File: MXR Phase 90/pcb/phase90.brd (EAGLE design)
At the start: 59 x 87.8 mm, 58 parts, among them IC1 TL072, IC2 TL074, J1 POWER_JACK, Q1 2N5457, Q2 2N5457, Q3 2N5457, Q4 2N5457, Q5 2N3906-, X1 2510-

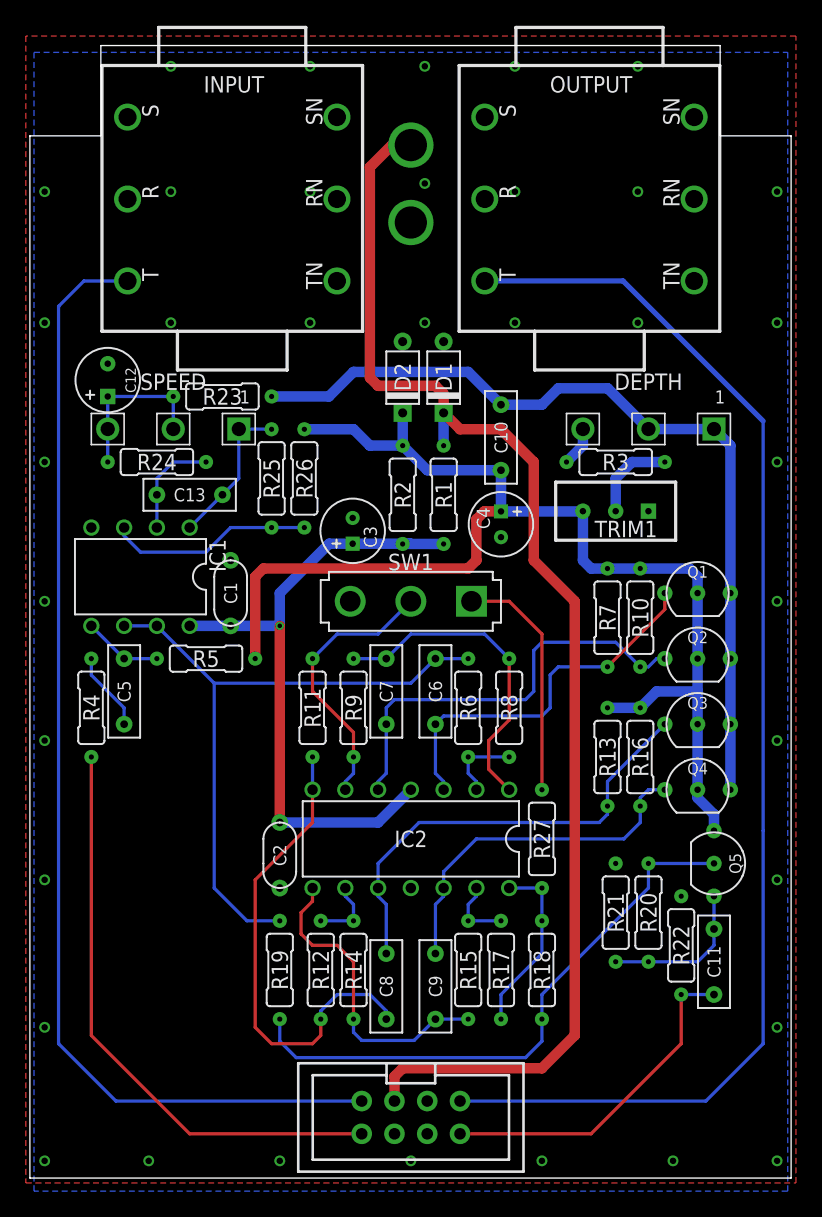
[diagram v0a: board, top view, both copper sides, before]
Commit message: 20171216
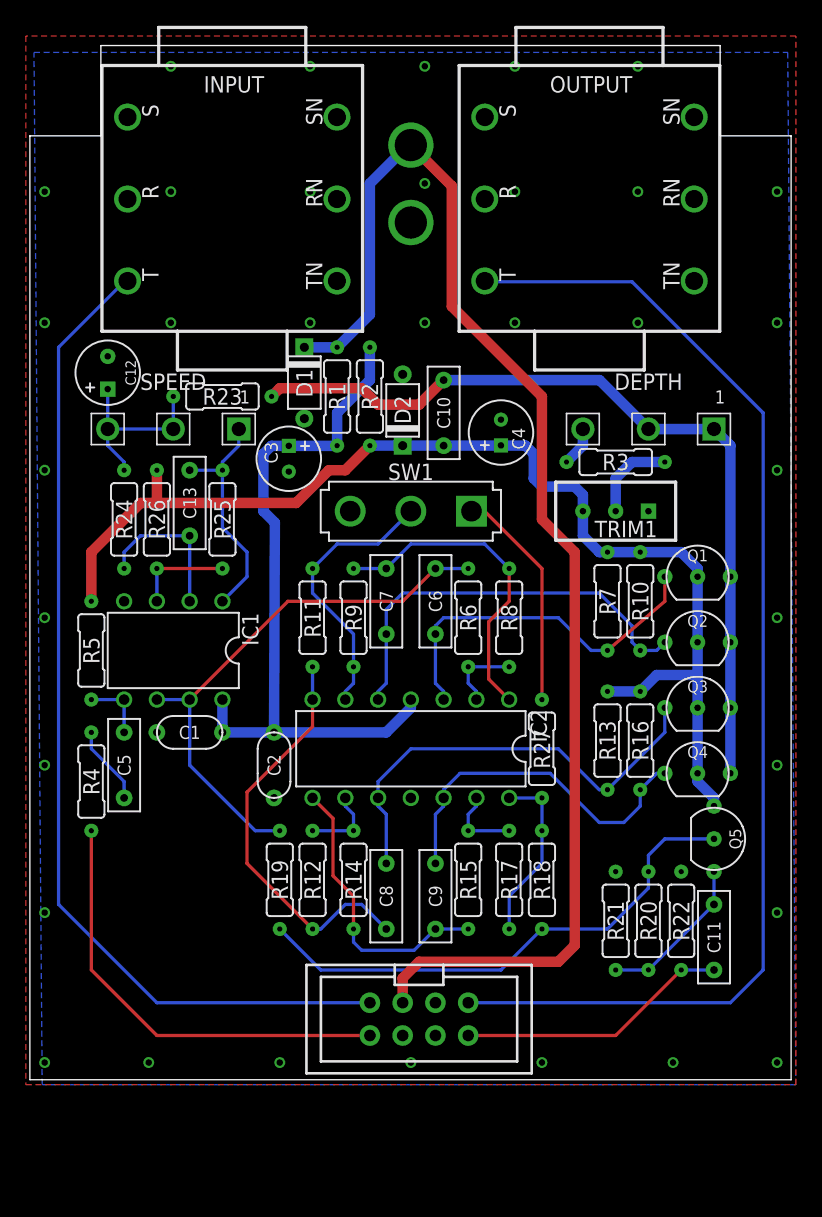
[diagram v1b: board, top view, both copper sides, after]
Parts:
- moved R26 11.9 mm to (9.53, 36.2)
- moved C1 11.3 mm to (12.1, 19.7), turned to 180 degrees
- moved R1 11.2 mm to (23.5, 45.7)
- moved D1 10.8 mm to (21.0, 46.8), turned to 270 degrees
- moved R5 8.91 mm to (4.45, 26.0), turned to 90 degrees
- moved R2 8.03 mm to (26.0, 45.7), turned to 270 degrees
- moved X1 7.65 mm to (29.8, -2.54)
- moved C3 7.47 mm to (19.7, 40.9), turned to 270 degrees
- moved C4 7.11 mm to (36.2, 42.9), turned to 90 degrees
- moved R12 7.01 mm to (21.6, 8.26)
- moved R17 7.01 mm to (36.8, 8.26)
- moved C2 7.00 mm to (18.6, 17.1)
- moved R14 6.99 mm to (24.8, 8.26)
- moved R15 6.99 mm to (33.7, 8.26)
- moved R18 6.99 mm to (39.4, 8.26)
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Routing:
- net IN: track 45.7 -> 34.5 mm
- net N$2: track 88.6 -> 77.9 mm
- net N$6: track 51.3 -> 42.5 mm
- net VB: track 99.0 -> 90.2 mm
- net N$15: track 15.9 -> 7.62 mm
- net N$4: track 99.7 -> 92.9 mm
- net N$19: track 11.8 -> 18.0 mm
- net N$14: track 37.3 -> 31.8 mm
- net OUT: track 26.4 -> 21.2 mm
- net N$24: track 45.4 -> 40.7 mm
- net N$26: track 8.15 -> 12.0 mm
- net VR: track 51.5 -> 55.2 mm, vias 1 -> 0
- net +9V: track 102.0 -> 104.3 mm
- net N$18: track 24.2 -> 22.3 mm
- net VA: track 66.4 -> 64.7 mm
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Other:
- board size 59 x 87.8 mm -> 59 x 80.2 mm
